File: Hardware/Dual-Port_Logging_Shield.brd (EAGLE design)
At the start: 22.9 x 58.4 mm, 115 parts, among them IC1 USB224X_2241, J2 MICRO-SD-PUSH-PUSH-EXT-PIN, J3 AVR_SPI_PROG_3X2TESTPOINTS, J4 THING_PLUS, Q1 20V/4.2A/52mΩ/1.4W, Q2 20V/0.2A/8MHz/1.2Ω/1Vth, Q3 20V/4.2A/52mΩ/1.4W, Q4 20V/4.2A/52mΩ/1.4W, Q6 20V/4.2A/52mΩ/1.4W, U1 3.3V, U2 74HC4066_QUAD_BILATERAL_SWITC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, U3 ATTINY841-ARDUINO_QFN20M1, U4 74HC4066_QUAD_BILATERAL_SWITC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, U5 74HC4066_QUAD_BILATERAL_SWITC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, U6 24C04, Y1 24MHz

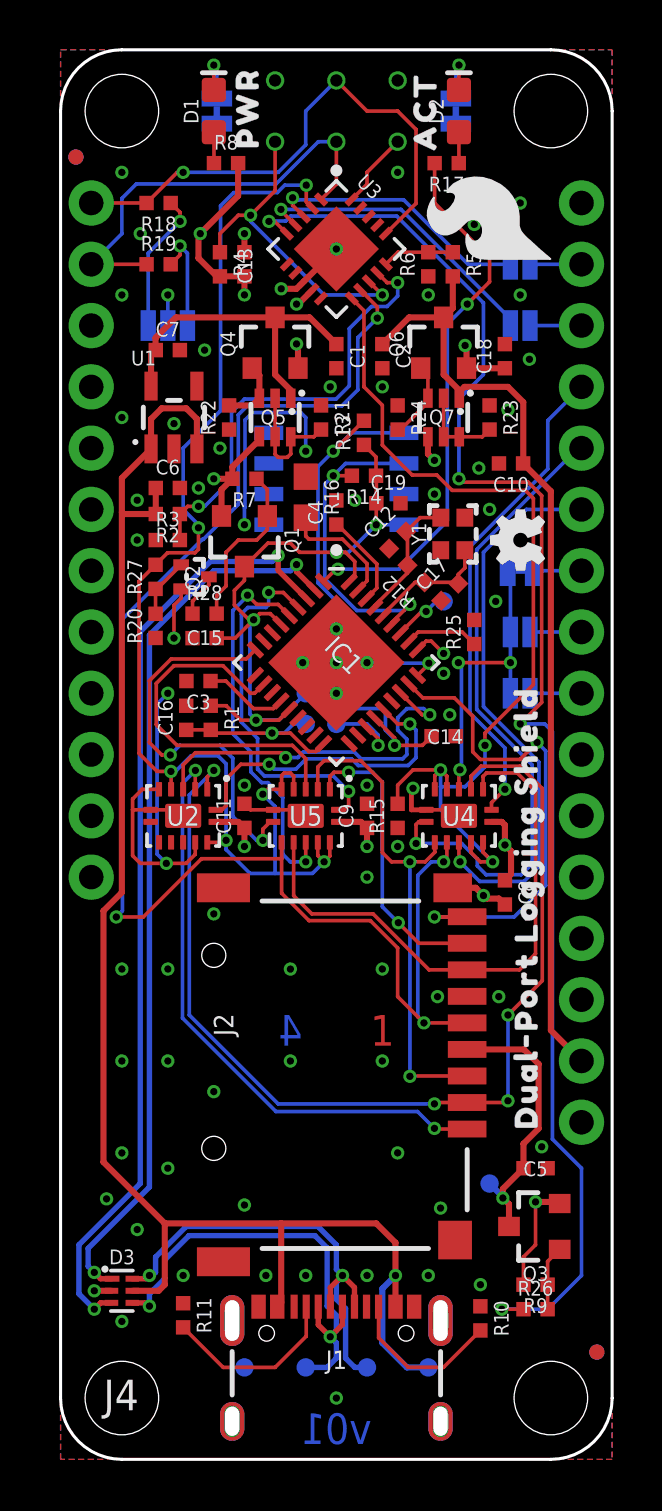
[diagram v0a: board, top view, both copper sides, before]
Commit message: Add v10 hardware files
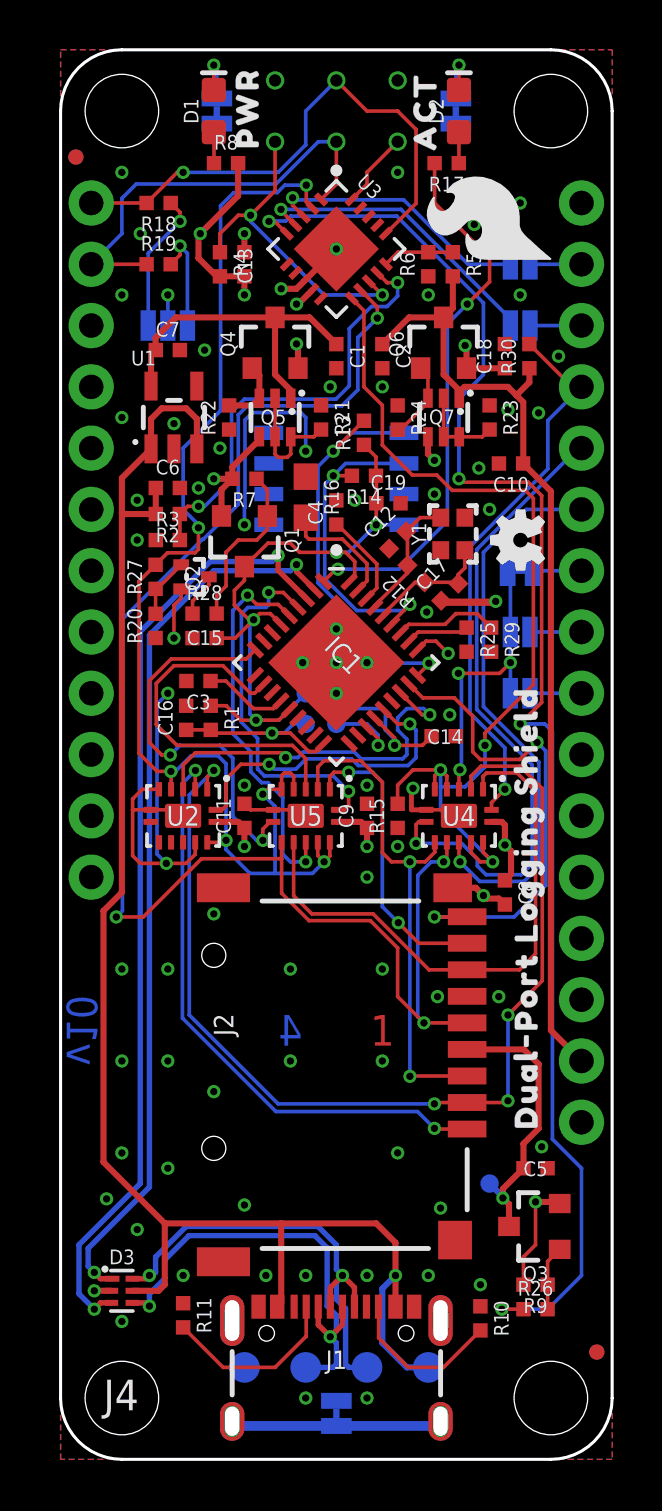
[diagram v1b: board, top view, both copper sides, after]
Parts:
- removed SD_WP: TEST-POINT3, SparkFun-Connectors:PAD.03X.03
- added R29, R30: 10k, SparkFun-Resistors:0402-TIGHT
- added SH: JUMPER-SMT_2_NC_TRACE_SILK, SparkFun-Jumpers:SMT-JUMPER_2_NC_TRACE_SILK
- added U$20: (no value), output:#SH#0
- added U$21: (no value), output:G0
- added U$22: (no value), output:V0
- added U$23: (no value), output:D#0
- added U$25: (no value), output:D#1
- D+, D-, GND, V_USB: value TEST-POINT3 -> TEST-POINT3X5; device SparkFun-Connectors:PAD.03X.03 -> SparkFun-Connectors:PAD.03X.05
- IC1: value USB224X_2241 -> USB224X_2241_V04; device USB224x:36-QFN -> SparkFun-IC-Special-Function:36-QFN
- R21, R23: value 10k -> 100k
- R22, R24: value 47k -> 1M
- U2, U4, U5: device 74HC4066:14-QFN -> SparkFun-IC-Logic:14-QFN
- moved R25 0.45 mm to (16.8, 34.0), turned to 270 degrees
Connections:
- removed net SD_WP: IC1.30, SD_WP.1
- new net N$12: J1.SHLD1, J1.SHLD2, J1.SHLD3, J1.SHLD4, SH.1
- new net N$20: IC1.30, R29.1
- net 3.3V: now also R30.1
- net GND: now also R29.2, SH.2
- net POCI: now also R30.2
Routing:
- net N$12: track 0.00 -> 17.2 mm
- net N$20: track 0.00 -> 4.33 mm
- net POCI: track 20.3 -> 23.2 mm
- net GND: track 44.1 -> 46.6 mm, vias 75 -> 77
- net SD_WP: track 2.33 -> 0.00 mm, vias 1 -> 0
- net 3.3V: track 40.0 -> 41.4 mm
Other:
- board text added: "v10"
- board text removed: "v01"
